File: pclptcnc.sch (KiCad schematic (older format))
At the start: 248 parts, among them P1 ARK825A-3, P3 ARK825A-4, P4 ARK825A-3, P5 ARK825A-3, P6 ARK825A-3, P7 ARK825A-3, P8 ARK825A-3, Q1 BC807-40, Q10 BC807-40, Q11 BC807-40, Q12 BC807-40, Q13 BC807-40, Q14 BC807-40, Q15 BC807-40, Q16 BC807-40, Q17 BC807-40, Q18 BC807-40, Q2 BC807-40, Q3 BC807-40, Q4 BC807-40, Q5 BC807-40, Q6 BC807-40, Q7 BC807-40, Q8 BC807-40, Q9 BC807-40, U1 74LVC1G3157GW, U10 SN74LVC2G17, U11 74HCT14, U12 SN74LVC2G17, U13 74HCT14, U2 HCPL2630, U3 HCPL2630, U4 HCPL2630, U5 HCPL2630, U6 HCPL2630, U7 HCPL2630, U8 74HCT14, U9 74HCT14, j1 DB25, j2 DB25

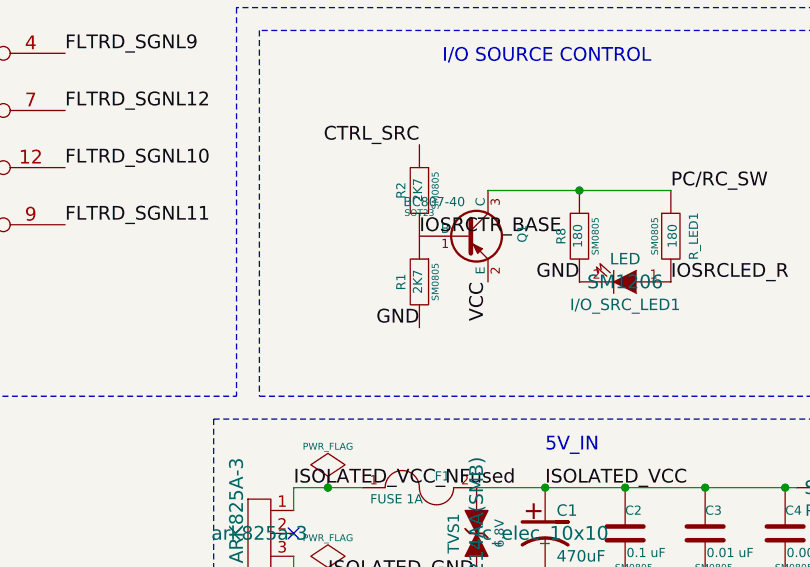
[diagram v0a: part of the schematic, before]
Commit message: version 0.2a completed
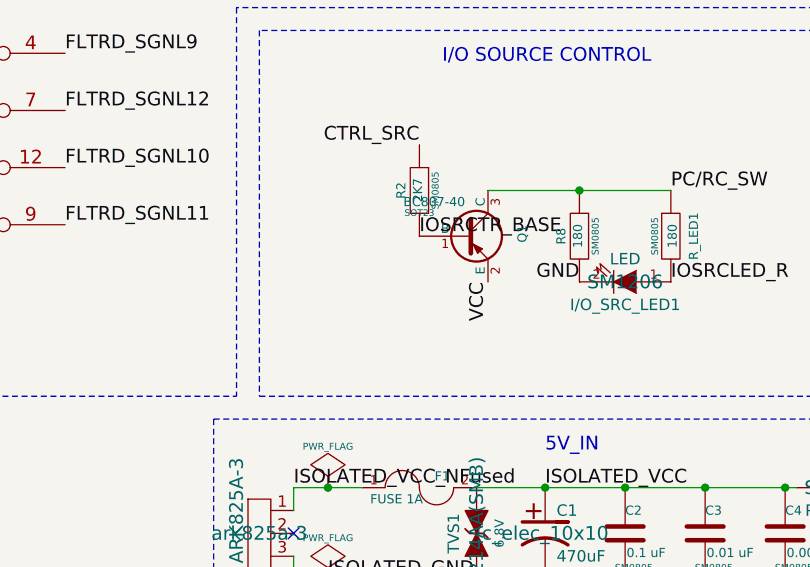
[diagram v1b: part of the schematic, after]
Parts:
- removed R1: 2K7, SM0805, symbol R_SFP
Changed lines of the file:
@@
 Text Label 5950 4150 2    60   ~ 0
 RC_SW_INV
-$Comp
-L BC807-40 Q1
-U 1 1 526C7C8B
-P 5900 5950
-F 0 "Q1" V 6150 6000 40  0000 R CNN
-F 1 "BC807-40" H 5900 6100 40  0000 R CNN
-F 2 "SOT23" H 5700 6052 29  0000 C CNN
-F 3 "~" H 5900 5950 60  0000 C CNN
-	1    5900 5950
-	1    0    0    -1
-$EndComp
-$Comp
-L R_SFP R1
-U 1 1 526C7CA0
-P 5700 6150
-F 0 "R1" V 5780 6150 40  0000 C CNN
-F 1 "2K7" V 5707 6151 40  0000 C CNN
-F 2 "SM0805" V 5630 6150 30  0000 C CNN
-F 3 "~" H 5700 6150 30  0000 C CNN
-	1    5700 6150
-	-1   0    0    -1
-$EndComp
-Text Label 5700 6350 2    60   ~ 0
-GND
 NoConn ~ 21850 11400
 NoConn ~ 20350 11400
@@
 	1    0    0    -1
 $EndComp
+$Comp
+L BC807-40 Q1
+U 1 1 526C7C8B
+P 5900 5950
+F 0 "Q1" V 6150 6000 40  0000 R CNN
+F 1 "BC807-40" H 5900 6100 40  0000 R CNN
+F 2 "SOT23" H 5700 6052 29  0000 C CNN
+F 3 "~" H 5900 5950 60  0000 C CNN
+	1    5900 5950
+	1    0    0    -1
+$EndComp
